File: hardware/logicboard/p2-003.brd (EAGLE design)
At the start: 72 x 72 mm, 67 parts, among them IC1 74LS06N, IC11 74LS153D, IC12 LTC485S, IC13 LTC485S, IC2 4066N, J1 MKR, J11 Qwiic, J12 Qwiic, J13 Qwiic, J14 Qwiic, J2 GPIO, J3 Vcc, J4 RLY, J5 SPI, J6 LED, K1 G5V1, T1 2SC1815, U1 DS18B20

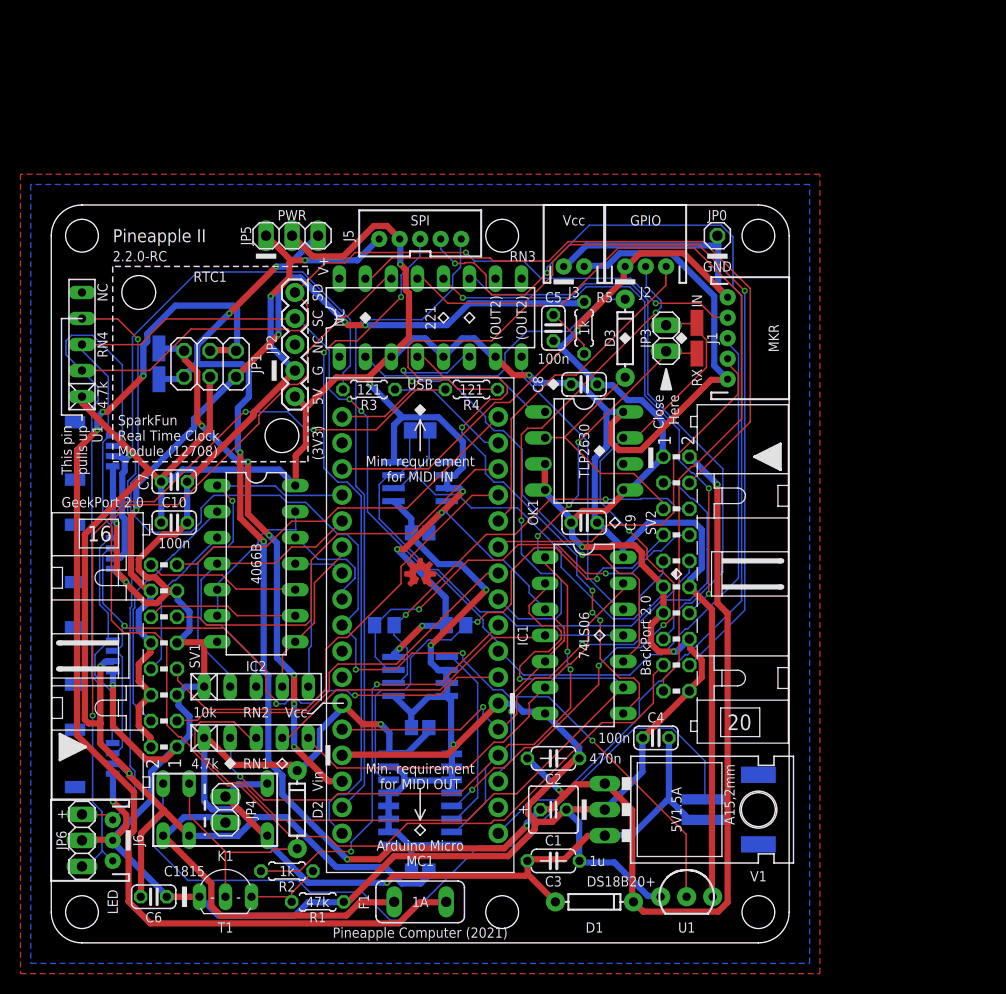
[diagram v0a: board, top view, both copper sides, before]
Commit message: Very rough but should be okay.
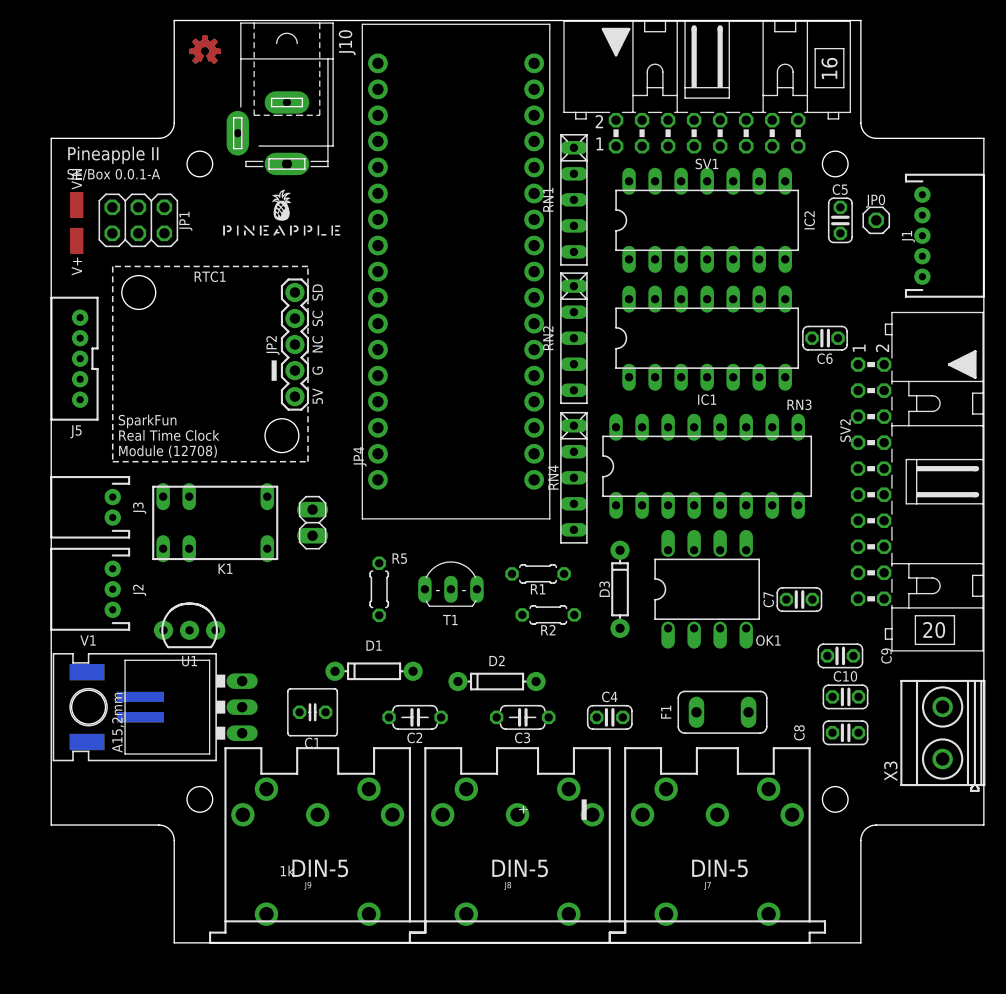
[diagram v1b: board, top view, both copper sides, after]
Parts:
- removed C11, C12, C13: 10n, rcl:C2012
- removed IC11: 74LS153D, 74xx-us:SO16
- removed IC12, IC13: LTC485S, linear-technology:SOIC8
- removed IN, RX: (no value), wirepad:SMD1,27-2,54
- removed J11, J12, J13, J14: Qwiic, SparkFun-Connectors:1X04_1MM_RA
- removed J6: LED, SparkFun-Connectors:JST-3-PTH
- removed JP3: MPXJMP, pinhead:1X02
- removed JP5: D5V, pinhead:1X03
- removed JP6: LED, pinhead:1X03
- removed R11: 10k, rcl:M2012
- removed R12, R13: 120, rcl:M2012
- removed R3, R4: 120, resistor:0204/5
- added J10: (no value), con-jack:SPC4077
- added J7, J8, J9: DIN5, SparkFun-Connectors:DIN5-RA-PTH
- added X3: MKDSN1,5/2-5,08, con-phoenix-508:MKDSN1,5/2-5,08
- moved C6 85.2 mm to (75.5, 59.0)
- moved SV1 73.6 mm to (64.0, 79.0), turned to 0 degrees
- moved C10 67.7 mm to (77.5, 24.0)
- moved J4 63.3 mm to (5.00, 23.0), turned to 270 degrees
- moved C7 62.1 mm to (73.0, 33.5)
- moved RN1 61.0 mm to (51.0, 72.5), turned to 270 degrees
- moved J2 60.8 mm to (6.00, 34.5), turned to 90 degrees
- moved IC2 55.3 mm to (64.0, 70.5), turned to 0 degrees
- moved LOGO1 55.2 mm to (15.0, 87.0)
- moved U1 55.0 mm to (13.5, 30.5)
- moved J3 50.8 mm to (6.00, 42.5), turned to 90 degrees
- moved RN4 49.7 mm to (51.0, 45.4), turned to 270 degrees
- moved RN2 46.0 mm to (51.0, 59.0), turned to 270 degrees
- moved V1 44.1 mm to (14.8, 23.0), turned to 90 degrees
- moved C8 42.5 mm to (77.5, 20.5)
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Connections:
- removed net LED0A: J6.1, JP6.1, R4.1
- removed net LED1A: J6.3, JP6.3, R3.1
- removed net MIN: IC11.5, IN.1, JP3.2, OK1.7
- removed net MRX: IC11.6, IC12.1
- net GND: now also X3.1; no longer C11.2, C12.2, C13.2, IC11.1, IC11.10, IC11.11, IC11.12, IC11.13, IC11.15, IC11.2, IC11.3, IC11.4, IC11.8, IC12.2, IC12.3, IC12.4, IC12.5, IC13.5, J11.1, J12.1, J13.1, J14.1, J6.2, JP5.1, JP6.2
- net LED0: no longer R4.2
- net LED1: no longer R3.2
- net MRX+: no longer IC12.6, R12.1
- net MRX-: no longer IC12.7, R12.2
- net MRXDTCT: no longer IC11.14, R11.1
- net MTX+: no longer IC13.6, R13.1
- net MTX-: no longer IC13.7, R13.2
- net RX: now also OK1.7; no longer IC11.7, JP3.1, RX.1
- net SCL: no longer J11.4, J12.4, J13.4, J14.4
- net SDA: no longer J11.3, J12.3, J13.3, J14.3
- net TX: no longer IC13.4
- net V+: now also X3.2; no longer JP5.3
- net VCC: no longer C11.1, C12.1, C13.1, IC11.16, IC12.8, IC13.2, IC13.3, IC13.8, J11.2, J12.2, J13.2, J14.2, JP5.2, R11.2
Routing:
- net GND: track 437.7 -> 0.00 mm, vias 12 -> 0
- net VCC: track 416.2 -> 0.00 mm, vias 12 -> 0
- net SDA: track 198.4 -> 0.00 mm, vias 5 -> 0
- net V+: track 181.3 -> 0.00 mm, vias 8 -> 0
- net SCL: track 160.7 -> 0.00 mm, vias 2 -> 0
- net MTSND: track 125.3 -> 0.00 mm
- net THS: track 110.8 -> 0.00 mm, vias 4 -> 0
- net VOUT: track 110.5 -> 0.00 mm, vias 3 -> 0
- net MOSI: track 105.9 -> 0.00 mm, vias 2 -> 0
- net LED0: track 101.2 -> 0.00 mm
- net RX: track 95.2 -> 0.00 mm, vias 6 -> 0
- net VCC/2: track 87.8 -> 0.00 mm, vias 4 -> 0
- net LED1A: track 85.0 -> 0.00 mm
- net NMTRTN: track 84.0 -> 0.00 mm, vias 1 -> 0
- net LED0A: track 77.0 -> 0.00 mm, vias 3 -> 0
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- removed copper zone on layer 1, net GND
- removed copper zone on layer 16, net GND
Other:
- board size 72 x 72 mm -> 91 x 90 mm
- board text added: "SE/Box 0.0.1-A"
- board text removed: "(3V3)"
- board text removed: "(OUT2)"
- board text removed: "*Cut pull-up R to install LM35"
- board text removed: "*Cut this pin to use LM35"
- board text removed: "100n"
- board text removed: "10k"
- board text removed: "121"
- board text removed: "1A"
- board text removed: "1u"
- board text removed: "2.2.0-RC"
- board text removed: "221"
- board text removed: "3V3"
- board text removed: "4.7k"
- board text removed: "4066B"
- board text removed: "470n"
- board text removed: "47k"
- board text removed: "5V1.5A"
- board text removed: "74153"
- board text removed: "74LS06"
- board text removed: "Arduino Micro"
- board text removed: "BackPort 2.0"
- board text removed: "C"
- board text removed: "C1815"
- board text removed: "Close"
- board text removed: "Close Here"
- board text removed: "D7"
- board text removed: "DS18B20+"
- board text removed: "Don't Close"
- board text removed: "Ext. V+"
- board text removed: "G1"
- board text removed: "G2"
- board text removed: "GND"
- board text removed: "GPIO"
- board text removed: "GeekPort 2.0"
- board text removed: "I"
- board text removed: "IN-RX"
- board text removed: "Insulating Tape Here"
- board text removed: "LED"
- board text removed: "LED0"
- board text removed: "LED1"
- board text removed: "LTC485"
- board text removed: "MC1"
- board text removed: "MKR"
- board text removed: "Min. requirement for MIDI IN"
- board text removed: "Min. requirement for MIDI OUT"
- board text removed: "O"
- board text removed: "OUT2"
- board text removed: "Open JP1"
- board text removed: "PWR"
- board text removed: "Pineapple Computer (2021)"
- board text removed: "Qwiic/5V"
- board text removed: "RLYJMP"
- board text removed: "RTN"
- board text removed: "RX"
- board text removed: "Relay"
- board text removed: "SCL"
- board text removed: "SDA"
- board text removed: "SND"
- board text removed: "SPI"
- board text removed: "TLP2630"
- board text removed: "TX"
- board text removed: "This pin pulls up U1"
- board text removed: "U1"
- board text removed: "USB"
- board text removed: "V"
- board text removed: "V+"
- board text removed: "Vcc"
- board text removed: "Vcc/2"
- board text removed: "Vin"
- board text removed: "Vin (MC)"
- board text removed: "Vout"
- board text removed: "Vout (Reg)"
- board text removed: "Voutraw"
- board text removed: "You can istall LM35* instead of DS18B20+"
